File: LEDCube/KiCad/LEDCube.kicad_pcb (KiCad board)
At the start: 2 copper layers, 70 x 50 mm, 9 parts, among them J1 BARREL_JACK, J2 ICSP HEADER, J3 TO_ANODES, J4 TO_CATHODES, U1 ATMEGA16-16PU, U2 LM7805, U3 ULN2803A

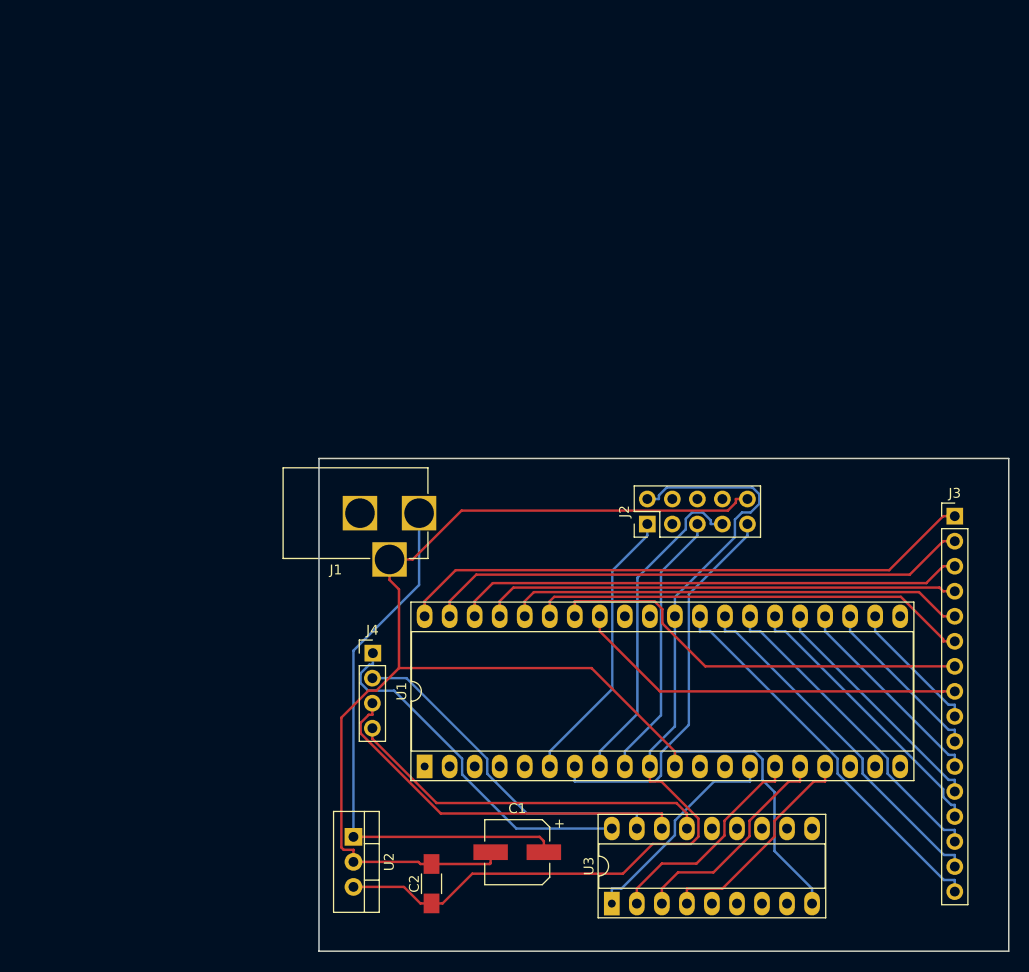
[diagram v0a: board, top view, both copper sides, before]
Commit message: Add files via upload
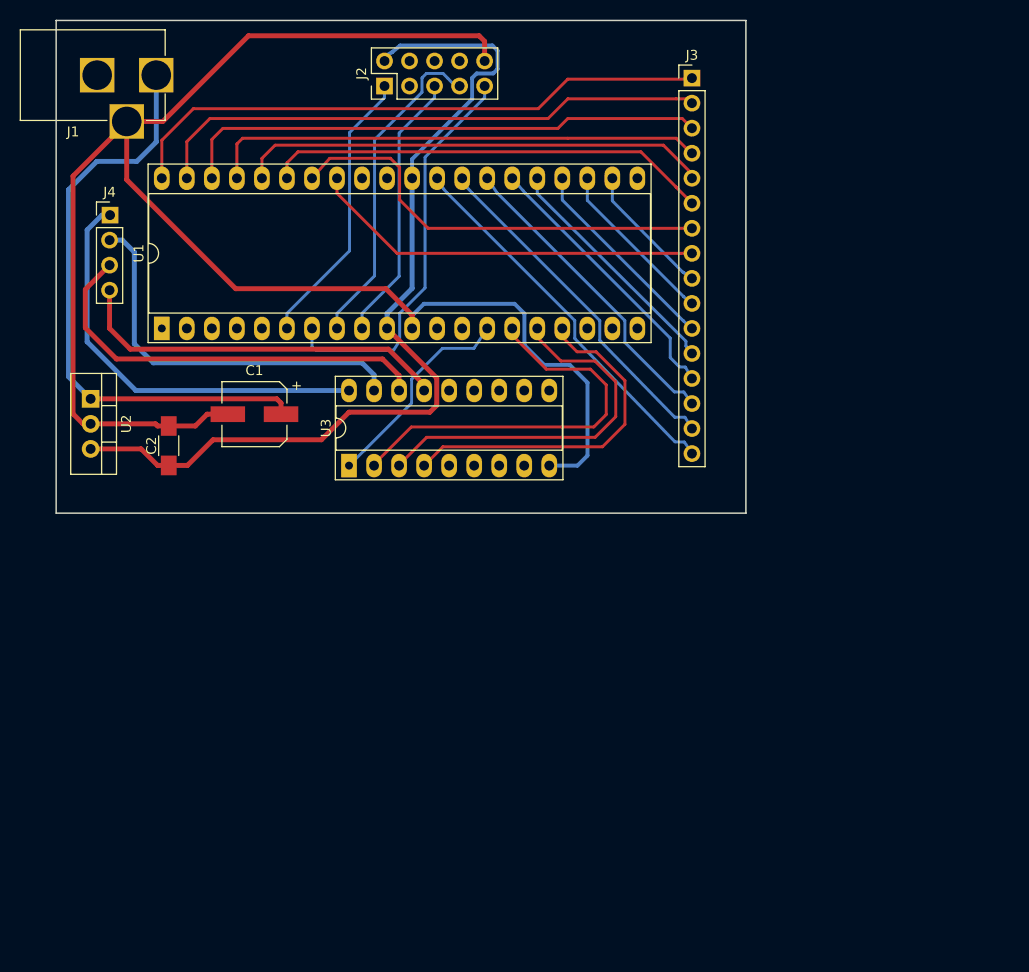
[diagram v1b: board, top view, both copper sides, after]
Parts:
- moved U1 51.8 mm to (80.1, 87.8)
- moved C1 51.8 mm to (89.5, 96.5)
- moved J1 51.8 mm to (79.6, 62.1)
- moved J2 51.8 mm to (102.7, 63.2)
- moved J3 51.8 mm to (133.9, 62.5)
- moved J4 51.8 mm to (74.8, 76.3)
- moved C2 51.8 mm to (80.8, 99.8)
- moved U2 51.8 mm to (72.9, 95.0)
- moved U3 51.8 mm to (99.1, 101.8)
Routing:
- net GND: track 149.8 -> 169.2 mm
- net Net-(U1-Pad15): track 22.5 -> 41.1 mm
- net Net-(U1-Pad16): track 22.5 -> 38.3 mm
- net Net-(U1-Pad17): track 22.5 -> 35.6 mm
- net Net-(J4-Pad1): track 36.3 -> 42.9 mm
- net Net-(J4-Pad2): track 34.9 -> 39.5 mm
- net +12V: track 56.2 -> 60.5 mm
- net Net-(J4-Pad3): track 39.2 -> 42.7 mm
- net Net-(J3-Pad3): track 51.7 -> 53.9 mm
- net Net-(J3-Pad4): track 48.4 -> 50.5 mm
- net Net-(J3-Pad2): track 55.3 -> 57.0 mm
- net Net-(J2-Pad3): track 1.42 -> 0.00 mm
- net Net-(J3-Pad1): track 58.9 -> 60.3 mm
- net Net-(J3-Pad5): track 46.6 -> 47.9 mm
- net Net-(J2-Pad9): track 39.7 -> 40.8 mm
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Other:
- net class Default: trace_width 0.25 -> 0.3
- rule trace_min: 0.25 -> 0.3
